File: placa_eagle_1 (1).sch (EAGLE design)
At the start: 19 parts, among them J1 CONN_0227-2021, J2 CONN_0427-2041, J3 CONN_0227-2021, J4 CONN_0227-2021, J5 CONN_0427-2041

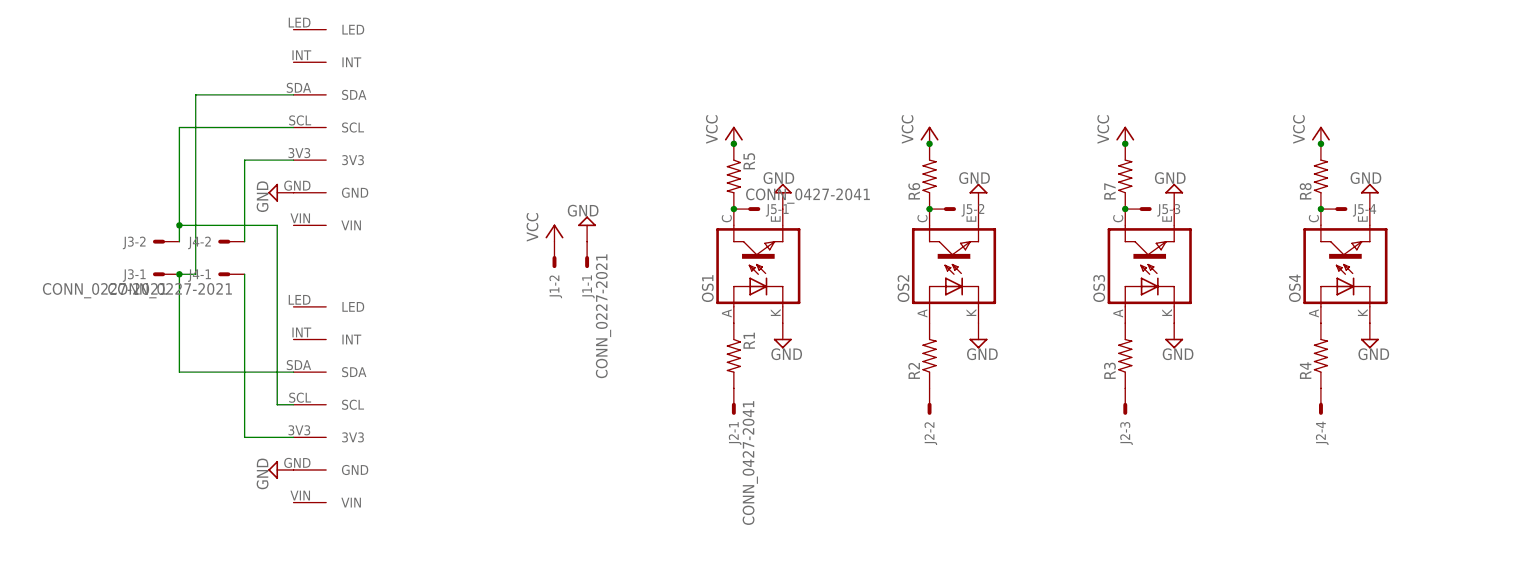
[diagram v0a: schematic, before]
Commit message: Placa ataulizada.
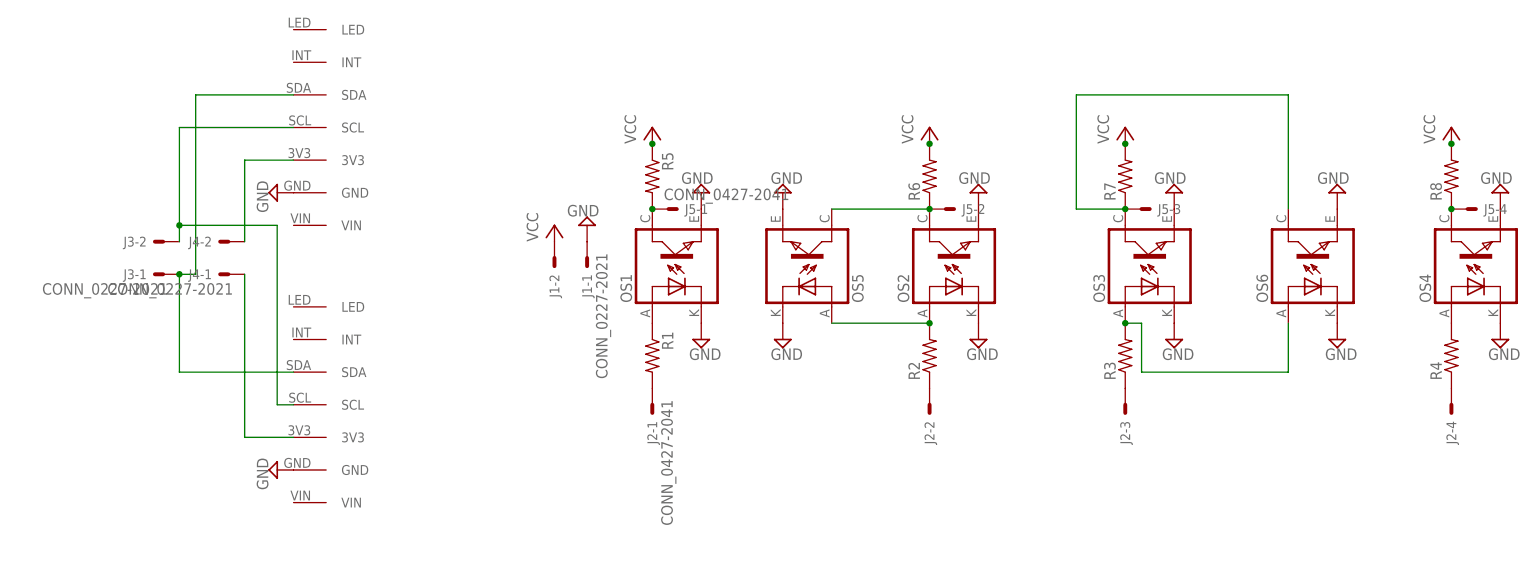
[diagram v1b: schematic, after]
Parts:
- added OS5, OS6: (no value), Robotica-IFRN-SC-sensores:TCRT5000
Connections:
- removed net N$2: OS2.ANODE, R2.2
- removed net N$3: OS3.ANODE, R3.2
- removed net N$6: J5-2.S, OS2.COLLECTOR, R6.1
- removed net N$7: J5-3.S, OS3.COLLECTOR, R7.1
- new net N$15: OS2.ANODE, OS5.ANODE, R2.2
- new net N$17: J5-2.S, OS2.COLLECTOR, OS5.COLLECTOR, R6.1
- new net N$19: OS3.ANODE, OS6.ANODE, R3.2
- new net N$20: J5-3.S, OS3.COLLECTOR, OS6.COLLECTOR, R7.1
- net GND: now also OS5.CATHODE, OS5.EMITTER, OS6.CATHODE, OS6.EMITTER
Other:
- moved on the sheet: J2-1, J2-4, J5-1, J5-4, OS1, OS4, R1, R4, R5, R8
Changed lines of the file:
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@@
 <layers>
 <layer number="1" name="Top" color="4" fill="1" visible="no" active="no"/>
+<layer number="2" name="Route2" color="1" fill="3" visible="no" active="no"/>
+<layer number="3" name="Route3" color="4" fill="3" visible="no" active="no"/>
+<layer number="4" name="Route4" color="1" fill="4" visible="no" active="no"/>
+<layer number="5" name="Route5" color="4" fill="4" visible="no" active="no"/>
+<layer number="6" name="Route6" color="1" fill="8" visible="no" active="no"/>
+<layer number="7" name="Route7" color="4" fill="8" visible="no" active="no"/>
+<layer number="8" name="Route8" color="1" fill="2" visible="no" active="no"/>
+<layer number="9" name="Route9" color="4" fill="2" visible="no" active="no"/>
+<layer number="10" name="Route10" color="1" fill="7" visible="no" active="no"/>
+<layer number="11" name="Route11" color="4" fill="7" visible="no" active="no"/>
+<layer number="12" name="Route12" color="1" fill="5" visible="no" active="no"/>
+<layer number="13" name="Route13" color="4" fill="5" visible="no" active="no"/>
+<layer number="14" name="Route14" color="1" fill="6" visible="no" active="no"/>
+<layer number="15" name="Route15" color="4" fill="6" visible="no" active="no"/>
 <layer number="16" name="Bottom" color="1" fill="1" visible="no" active="no"/>
 <layer number="17" name="Pads" color="2" fill="1" visible="no" active="no"/>
@@
 <part name="SUPPLY10" library="supply2" library_urn="urn:adsk.eagle:library:372" deviceset="GND" device=""/>
 <part name="SUPPLY11" library="supply2" library_urn="urn:adsk.eagle:library:372" deviceset="GND" device=""/>
+<part name="OS5" library="Robotica-IFRN-SC-sensores" deviceset="TCRT5000" device=""/>
+<part name="OS6" library="Robotica-IFRN-SC-sensores" deviceset="TCRT5000" device=""/>
+<part name="SUPPLY14" library="supply2" library_urn="urn:adsk.eagle:library:372" deviceset="GND" device=""/>
+<part name="SUPPLY15" library="supply2" library_urn="urn:adsk.eagle:library:372" deviceset="GND" device=""/>
+<part name="SUPPLY16" library="supply2" library_urn="urn:adsk.eagle:library:372" deviceset="GND" device=""/>
+<part name="SUPPLY19" library="supply2" library_urn="urn:adsk.eagle:library:372" deviceset="GND" device=""/>
 </parts>
 <sheets>
@@
 </plain>
 <instances>
-<instance part="OS1" gate="OS" x="7.62" y="83.82" rot="R90"/>
+<instance part="OS1" gate="OS" x="-5.08" y="83.82" rot="R90"/>
 <instance part="OS2" gate="OS" x="38.1" y="83.82" rot="R90"/>
 <instance part="OS3" gate="OS" x="68.58" y="83.82" rot="R90"/>
-<instance part="OS4" gate="OS" x="99.06" y="83.82" rot="R90"/>
-<instance part="R1" gate="G$1" x="5.08" y="68.58" rot="R270"/>
+<instance part="OS4" gate="OS" x="119.38" y="83.82" rot="R90"/>
+<instance part="R1" gate="G$1" x="-7.62" y="68.58" rot="R270"/>
 <instance part="R2" gate="G$1" x="35.56" y="68.58" rot="R90"/>
 <instance part="R3" gate="G$1" x="66.04" y="68.58" rot="R90"/>
-<instance part="R4" gate="G$1" x="96.52" y="68.58" rot="R90"/>
-<instance part="R5" gate="G$1" x="5.08" y="96.52" rot="R270"/>
+<instance part="R4" gate="G$1" x="116.84" y="68.58" rot="R90"/>
+<instance part="R5" gate="G$1" x="-7.62" y="96.52" rot="R270"/>
 <instance part="R6" gate="G$1" x="35.56" y="96.52" rot="R90"/>
 <instance part="R7" gate="G$1" x="66.04" y="96.52" rot="R90"/>
-<instance part="R8" gate="G$1" x="96.52" y="96.52" rot="R90"/>
-<instance part="P+1" gate="VCC" x="5.08" y="104.14"/>
+<instance part="R8" gate="G$1" x="116.84" y="96.52" rot="R90"/>
+<instance part="P+1" gate="VCC" x="-7.62" y="104.14"/>
 <instance part="P+2" gate="VCC" x="35.56" y="104.14"/>
 <instance part="P+3" gate="VCC" x="66.04" y="104.14"/>
-<instance part="P+4" gate="VCC" x="96.52" y="104.14"/>
-<instance part="SUPPLY1" gate="GND" x="12.7" y="71.12"/>
+<instance part="P+4" gate="VCC" x="116.84" y="104.14"/>
+<instance part="SUPPLY1" gate="GND" x="0" y="71.12"/>
 <instance part="SUPPLY2" gate="GND" x="43.18" y="71.12"/>
 <instance part="SUPPLY3" gate="GND" x="73.66" y="71.12"/>
-<instance part="SUPPLY4" gate="GND" x="104.14" y="71.12"/>
-<instance part="SUPPLY5" gate="GND" x="12.7" y="93.98" rot="R180"/>
+<instance part="SUPPLY4" gate="GND" x="124.46" y="71.12"/>
+<instance part="SUPPLY5" gate="GND" x="0" y="93.98" rot="R180"/>
 <instance part="SUPPLY6" gate="GND" x="43.18" y="93.98" rot="R180"/>
 <instance part="SUPPLY7" gate="GND" x="73.66" y="93.98" rot="R180"/>
-<instance part="SUPPLY8" gate="GND" x="104.14" y="93.98" rot="R180"/>
+<instance part="SUPPLY8" gate="GND" x="124.46" y="93.98" rot="R180"/>
 <instance part="J1" gate="-1" x="-17.78" y="83.82" rot="R270"/>
 <instance part="J1" gate="-2" x="-22.86" y="83.82" rot="R270"/>
-<instance part="J2" gate="-1" x="5.08" y="60.96" rot="R270"/>
+<instance part="J2" gate="-1" x="-7.62" y="60.96" rot="R270"/>
 <instance part="J2" gate="-2" x="35.56" y="60.96" rot="R270"/>
 <instance part="J2" gate="-3" x="66.04" y="60.96" rot="R270"/>
-<instance part="J2" gate="-4" x="96.52" y="60.96" rot="R270"/>
+<instance part="J2" gate="-4" x="116.84" y="60.96" rot="R270"/>
 <instance part="SUPPLY9" gate="GND" x="-17.78" y="88.9" rot="R180"/>
 <instance part="P+5" gate="VCC" x="-22.86" y="88.9"/>
-<instance part="J5" gate="-1" x="7.62" y="91.44"/>
+<instance part="J5" gate="-1" x="-5.08" y="91.44"/>
 <instance part="J5" gate="-2" x="38.1" y="91.44"/>
 <instance part="J5" gate="-3" x="68.58" y="91.44"/>
-<instance part="J5" gate="-4" x="99.06" y="91.44"/>
+<instance part="J5" gate="-4" x="119.38" y="91.44"/>
 <instance part="J3" gate="-1" x="-83.82" y="81.28" rot="R180"/>
 <instance part="J3" gate="-2" x="-83.82" y="86.36" rot="R180"/>
@@
 <instance part="SUPPLY10" gate="GND" x="-66.04" y="50.8" rot="R270"/>
 <instance part="SUPPLY11" gate="GND" x="-66.04" y="93.98" rot="R270"/>
+<instance part="OS5" gate="OS" x="17.78" y="83.82" rot="MR90"/>
+<instance part="OS6" gate="OS" x="93.98" y="83.82" rot="R90"/>
+<instance part="SUPPLY14" gate="GND" x="99.06" y="71.12"/>
+<instance part="SUPPLY15" gate="GND" x="99.06" y="93.98" rot="R180"/>
+<instance part="SUPPLY16" gate="GND" x="12.7" y="71.12"/>
+<instance part="SUPPLY19" gate="GND" x="12.7" y="93.98" rot="MR180"/>
 </instances>
 <busses>
@@
 </segment>
 </net>
-<net name="N$2" class="0">
-<segment>
-<pinref part="OS2" gate="OS" pin="ANODE"/>
-<pinref part="R2" gate="G$1" pin="2"/>
-</segment>
-</net>
-<net name="N$3" class="0">
-<segment>
-<pinref part="OS3" gate="OS" pin="ANODE"/>
-<pinref part="R3" gate="G$1" pin="2"/>
-</segment>
-</net>
 <net name="N$4" class="0">
 <segment>
@@
 <pinref part="R5" gate="G$1" pin="2"/>
 <pinref part="J5" gate="-1" pin="S"/>
-<junction x="5.08" y="91.44"/>
-</segment>
-</net>
-<net name="N$6" class="0">
-<segment>
-<pinref part="OS2" gate="OS" pin="COLLECTOR"/>
-<pinref part="R6" gate="G$1" pin="1"/>
-<pinref part="J5" gate="-2" pin="S"/>
-<junction x="35.56" y="91.44"/>
-</segment>
-</net>
-<net name="N$7" class="0">
-<segment>
-<pinref part="OS3" gate="OS" pin="COLLECTOR"/>
-<pinref part="R7" gate="G$1" pin="1"/>
-<pinref part="J5" gate="-3" pin="S"/>
-<junction x="66.04" y="91.44"/>
+<junction x="-7.62" y="91.44"/>
 </segment>
 </net>
@@
 <pinref part="R8" gate="G$1" pin="1"/>
 <pinref part="J5" gate="-4" pin="S"/>
-<junction x="96.52" y="91.44"/>
+<junction x="116.84" y="91.44"/>
 </segment>
 </net>
@@
 <pinref part="P+1" gate="VCC" pin="VCC"/>
 <pinref part="R5" gate="G$1" pin="1"/>
-<junction x="5.08" y="101.6"/>
+<junction x="-7.62" y="101.6"/>
 </segment>
 <segment>
@@
 <pinref part="P+4" gate="VCC" pin="VCC"/>
 <pinref part="R8" gate="G$1" pin="2"/>
-<junction x="96.52" y="101.6"/>
+<junction x="116.84" y="101.6"/>
 </segment>
 <segment>
@@
 <pinref part="J1" gate="-1" pin="S"/>
 <pinref part="SUPPLY9" gate="GND" pin="GND"/>
+</segment>
+<segment>
+<pinref part="OS6" gate="OS" pin="CATHODE"/>
+<pinref part="SUPPLY14" gate="GND" pin="GND"/>
+</segment>
+<segment>
+<pinref part="OS6" gate="OS" pin="EMITTER"/>
+<pinref part="SUPPLY15" gate="GND" pin="GND"/>
+</segment>
+<segment>
+<pinref part="OS5" gate="OS" pin="EMITTER"/>
+<pinref part="SUPPLY19" gate="GND" pin="GND"/>
+</segment>
+<segment>
+<pinref part="OS5" gate="OS" pin="CATHODE"/>
+<pinref part="SUPPLY16" gate="GND" pin="GND"/>
 </segment>
 </net>
@@
 </segment>
 </net>
+<net name="N$15" class="0">
+<segment>
+<pinref part="OS2" gate="OS" pin="ANODE"/>
+<pinref part="R2" gate="G$1" pin="2"/>
+<junction x="35.56" y="73.66"/>
+<pinref part="OS5" gate="OS" pin="ANODE"/>
+<wire x1="35.56" y1="73.66" x2="20.32" y2="73.66" width="0.1524" layer="91"/>
+</segment>
+</net>
+<net name="N$17" class="0">
+<segment>
+<pinref part="OS2" gate="OS" pin="COLLECTOR"/>
+<pinref part="R6" gate="G$1" pin="1"/>
+<pinref part="J5" gate="-2" pin="S"/>
+<junction x="35.56" y="91.44"/>
+<pinref part="OS5" gate="OS" pin="COLLECTOR"/>
+<wire x1="35.56" y1="91.44" x2="20.32" y2="91.44" width="0.1524" layer="91"/>
+</segment>
+</net>
+<net name="N$19" class="0">
+<segment>
+<pinref part="OS6" gate="OS" pin="ANODE"/>
+<wire x1="91.44" y1="73.66" x2="91.44" y2="66.04" width="0.1524" layer="91"/>
+<wire x1="91.44" y1="66.04" x2="68.58" y2="66.04" width="0.1524" layer="91"/>
+<wire x1="68.58" y1="66.04" x2="68.58" y2="73.66" width="0.1524" layer="91"/>
+<pinref part="OS3" gate="OS" pin="ANODE"/>
+<pinref part="R3" gate="G$1" pin="2"/>
+<wire x1="68.58" y1="73.66" x2="66.04" y2="73.66" width="0.1524" layer="91"/>
+<junction x="66.04" y="73.66"/>
+</segment>
+</net>
+<net name="N$20" class="0">
+<segment>
+<pinref part="OS6" gate="OS" pin="COLLECTOR"/>
+<wire x1="91.44" y1="91.44" x2="91.44" y2="109.22" width="0.1524" layer="91"/>
+<wire x1="91.44" y1="109.22" x2="58.42" y2="109.22" width="0.1524" layer="91"/>
+<pinref part="OS3" gate="OS" pin="COLLECTOR"/>
+<pinref part="R7" gate="G$1" pin="1"/>
+<pinref part="J5" gate="-3" pin="S"/>
+<junction x="66.04" y="91.44"/>
+<wire x1="58.42" y1="109.22" x2="58.42" y2="91.44" width="0.1524" layer="91"/>
+<wire x1="58.42" y1="91.44" x2="66.04" y2="91.44" width="0.1524" layer="91"/>
+</segment>
+</net>
